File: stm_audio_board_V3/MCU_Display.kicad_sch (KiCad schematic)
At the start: 16 parts, among them J10 USB_A, SW1 SW_SPST, U1 IS42S16100H-7TL, U7 STM32H723ZGTx, Y2 X1E0000210132

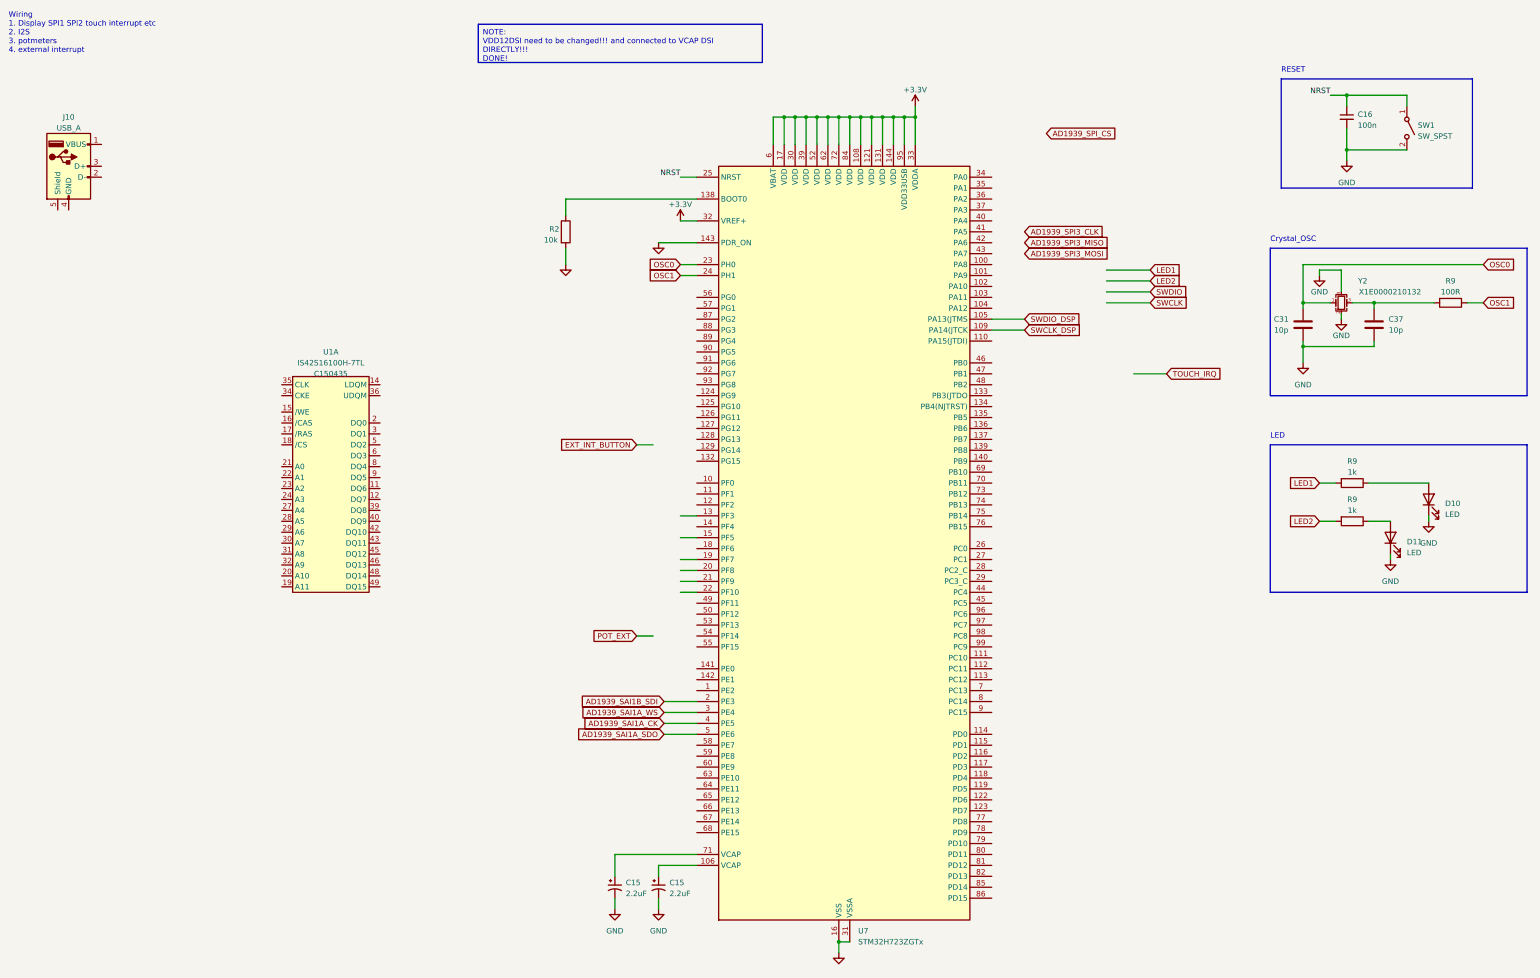
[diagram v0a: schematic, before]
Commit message: minor changes
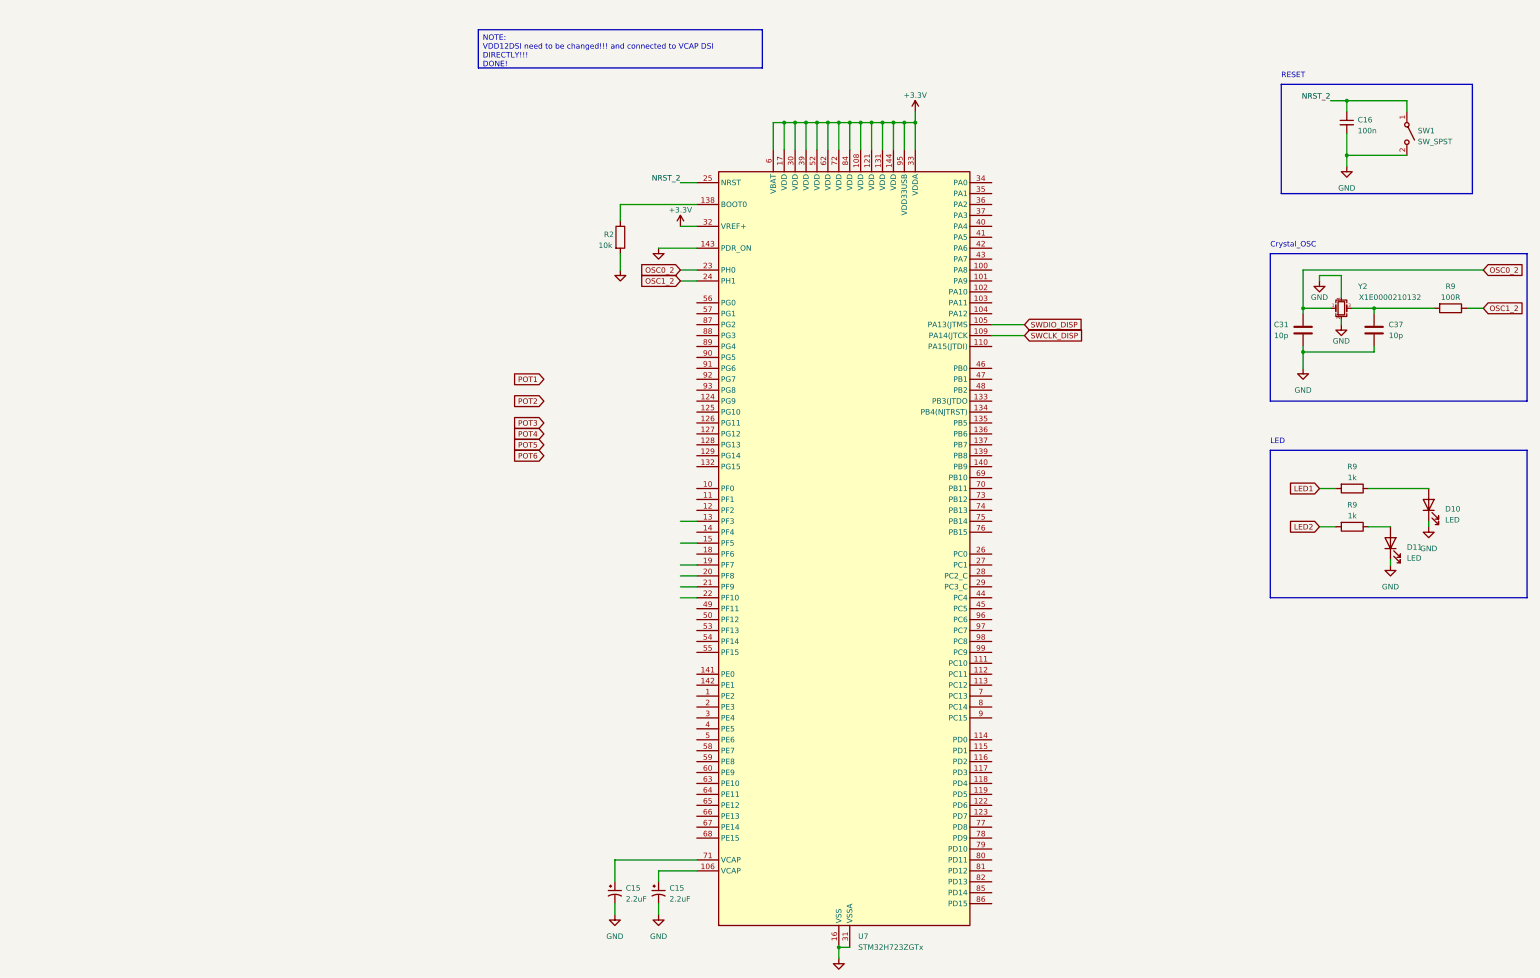
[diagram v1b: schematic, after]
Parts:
- removed C15 (x2): 2.2uF, Capacitor_SMD:C_0805_2012Metric_Pad1.18x1.45mm_HandSolder, symbol Device:C_Polarized_Small_US
- removed J10: USB_A, Connector_USB:USB_A_CONNFLY_DS1095-WNR0, symbol Connector:USB_A
- removed R9 (x2): 1k, Resistor_SMD:R_0603_1608Metric_Pad0.98x0.95mm_HandSolder, symbol Device:R
- removed R9: 100R, Resistor_SMD:R_0603_1608Metric, symbol Device:R
- removed U1: IS42S16100H-7TL, Library:TSOP-2-50-new, symbol stm_audio:IS42S16100H-7TL
- added C15 (x2): 2.2uF, Capacitor_SMD:C_0805_2012Metric_Pad1.18x1.45mm_HandSolder, symbol Device:C_Polarized_Small_US
- added R9 (x2): 1k, Resistor_SMD:R_0603_1608Metric_Pad0.98x0.95mm_HandSolder, symbol Device:R
- added R9: 100R, Resistor_SMD:R_0603_1608Metric, symbol Device:R
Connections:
- net GND: now also C15.2, C15.2
- net LED1: now also R9.2
- net LED2: now also R9.2
- net at D10.2 (A): now also R9.1
- net at C37.2, Y2.3: now also R9.2
- net at U7.71 (VCAP): now also C15.1
- net at D11.2 (A): now also R9.1
- net at U7.106 (VCAP): now also C15.1
- net AD1939_SAI1A_CK: no longer names the net of U7.4 (PE5)
- net AD1939_SAI1A_SDO: no longer names the net of U7.5 (PE6)
- net AD1939_SAI1A_WS: no longer names the net of U7.3 (PE4)
- net AD1939_SAI1B_SDI: no longer names the net of U7.2 (PE3)
- net NRST renamed NRST_2
- net OSC0 renamed OSC0_2
- net OSC1 renamed OSC1_2
- net OSC1_2: now also R9.1
- net SWCLK_DSP renamed SWCLK_DISP
- net SWDIO_DSP renamed SWDIO_DISP
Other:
- note removed: "Wiring 1. Display SPI1 SPI2 touch interrupt etc 2. I2S 3. potmeters 4. external interrupt"
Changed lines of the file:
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@@
 (kicad_sch (version 20230121) (generator eeschema)
-  (paper "A3")
+  (paper "A2")
